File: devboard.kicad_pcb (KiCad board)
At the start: 2 copper layers, 23 x 52 mm, 24 parts, among them J1 USB4105-GF-A, J2 Conn_01x08_Pin, J3 Conn_01x08_Pin, U1 STM32F411CEU6, U2 AP2120N-3.3TRG1, U3 USBLC6-2SC6Y

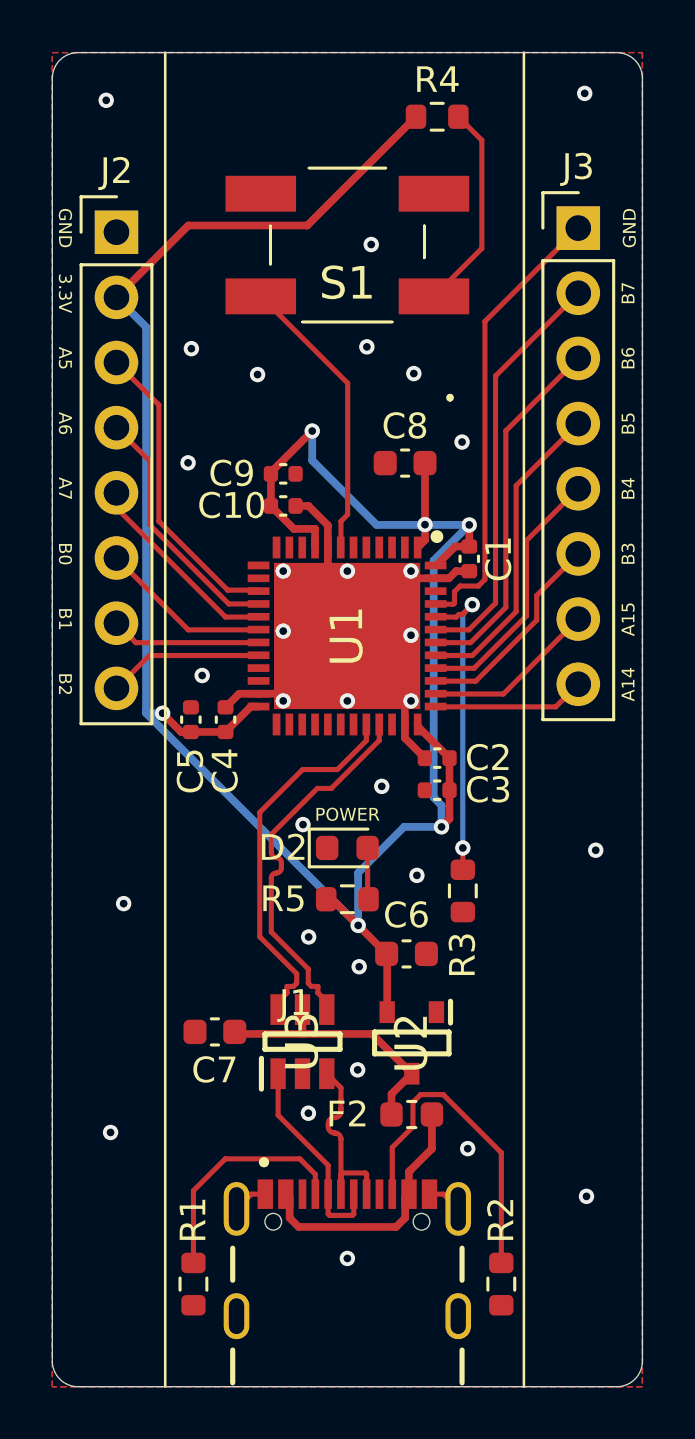
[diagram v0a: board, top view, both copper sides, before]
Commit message: Fixes
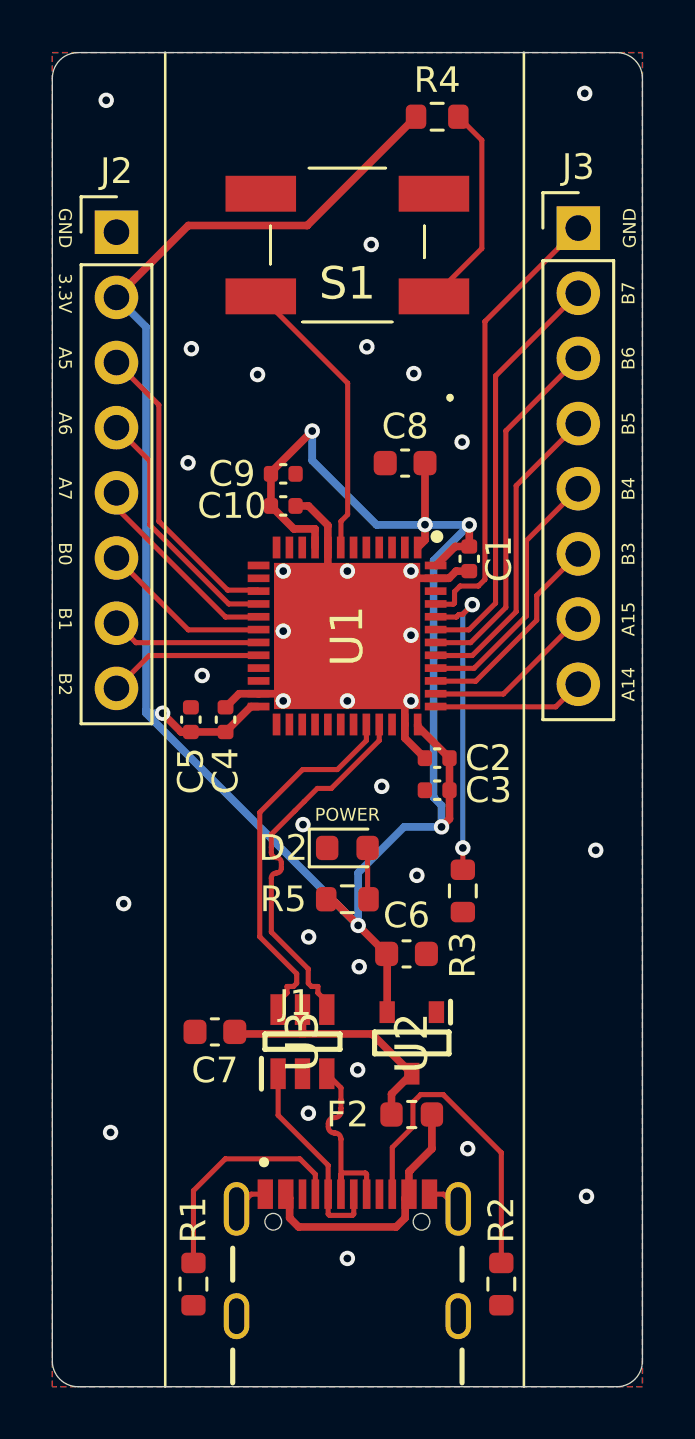
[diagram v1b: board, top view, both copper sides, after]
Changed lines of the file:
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@@
-		(net 33)
-		(net_name "GND")
-		(layer "F.Cu")
-		(hatch edge 0.5)
-		(connect_pads
-			(clearance 0.5)
-		)
-		(min_thickness 0.25)
-		(filled_areas_thickness no)
-		(fill yes
-			(thermal_gap 0.5)
-			(thermal_bridge_width 0.5)
-		)
-		(polygon
-			(pts
-				(xy 102 73) (xy 125 73) (xy 125 125) (xy 102 125)
-			)
-		)
-	)
-	(zone
 		(net 33)
 		(net_name "GND")
